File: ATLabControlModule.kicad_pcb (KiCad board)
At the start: 4 copper layers, 44 x 24 mm, 42 parts, among them J1 USB_Type_C_Receptacle, J2 Conn_ARM_SWD_TagConnect_TC2030, SW1 Kailh_Choc_V2_Brown, SW2 Kailh_Choc_V2_Brown, U1 STM32G0B1KEUx, U2 USBLC6-2P6, U3 MIC5317-3.3xM5, U4 SN74LVC1G17DBVRG4

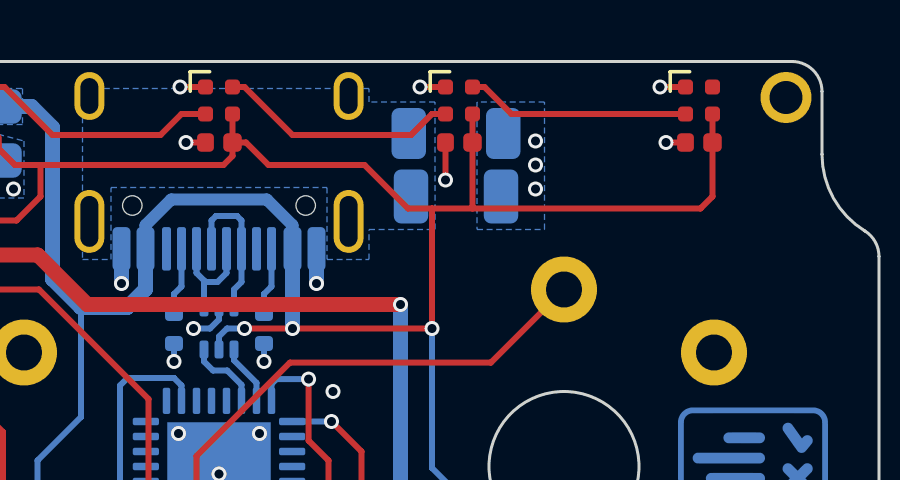
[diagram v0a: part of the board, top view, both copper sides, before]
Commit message: cleanup and add docs
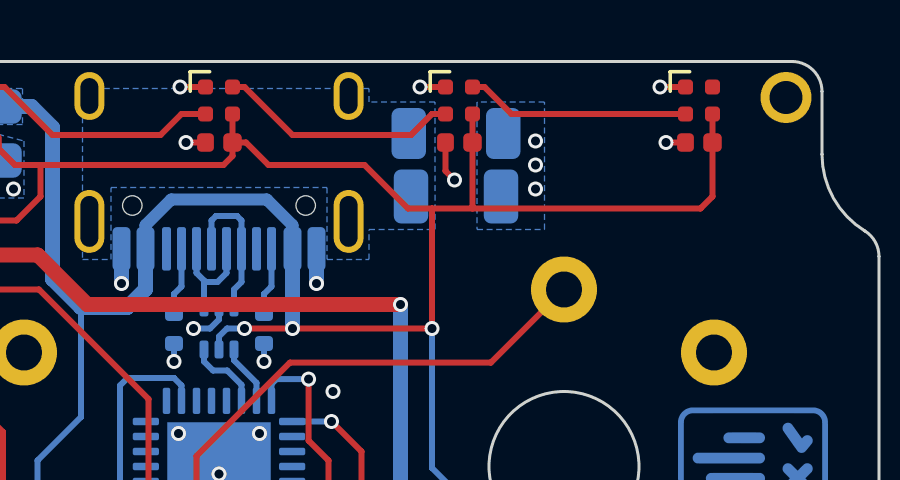
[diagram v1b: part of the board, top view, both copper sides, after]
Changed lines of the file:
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@@
 			)
 		)
-		(property "Datasheet" ""
+		(property "Datasheet" "https://www.lcsc.com/datasheet/C5149201.pdf"
 			(at 0 0 0)
 			(unlocked yes)
@@
 			)
 		)
-		(property "Description" ""
+		(property "Description" "RGB LED with integrated controller"
 			(at 0 0 0)
 			(unlocked yes)
@@
 			)
 		)
+		(property "Manufacturer" "OPSCO Optoelectronics"
+			(at 0 0 180)
+			(unlocked yes)
+			(layer "B.Fab")
+			(hide yes)
+			(effects
+				(font
+					(size 1 1)
+					(thickness 0.15)
+				)
+				(justify mirror)
+			)
+		)
+		(property "Manufacturer Part Number" "SK6812MINI-E"
+			(at 0 0 180)
+			(unlocked yes)
+			(layer "B.Fab")
+			(hide yes)
+			(effects
+				(font
+					(size 1 1)
+					(thickness 0.15)
+				)
+				(justify mirror)
+			)
+		)
+		(property "Distributor" "JLCPCB"
+			(at 0 0 180)
+			(unlocked yes)
+			(layer "B.Fab")
+			(hide yes)
+			(effects
+				(font
+					(size 1 1)
+					(thickness 0.15)
+				)
+				(justify mirror)
+			)
+		)
+		(property "Distributor Part Number" " C5149201"
+			(at 0 0 180)
+			(unlocked yes)
+			(layer "B.Fab")
+			(hide yes)
+			(effects
+				(font
+					(size 1 1)
+					(thickness 0.15)
+				)
+				(justify mirror)
+			)
+		)
 		(property ki_fp_filters "LED?SK6812MINI?E?3.2x2.8mm?P1.5mm*")
 		(sheetname "/")
 		(sheetfile "ATLabControlModule.kicad_sch")
+		(units
+			(unit
+				(name "A")
+				(pins "2" "3" "1" "4")
+			)
+		)
 		(attr smd)
 		(duplicate_pad_numbers_are_jumpers no)
@@
 			)
 		)
-		(property "Manufacturer" ""
+		(property "Manufacturer" "STMicroelectronics"
 			(at 0 0 270)
 			(unlocked yes)
@@
 			)
 		)
-		(property "Manufacturer Part Number" ""
+		(property "Manufacturer Part Number" "STM32G0B1KEU6"
 			(at 0 0 270)
 			(unlocked yes)
@@
 			)
 		)
-		(property "Distributor" ""
+		(property "Distributor" "Digikey"
 			(at 0 0 270)
 			(unlocked yes)
@@
 			)
 		)
-		(property "Distributor Part Number" ""
+		(property "Distributor Part Number" "497-STM32G0B1KEU6-ND"
 			(at 0 0 270)
 			(unlocked yes)
@@
 			)
 		)
-		(property "Datasheet" ""
+		(property "Datasheet" "https://www.lcsc.com/datasheet/C5149201.pdf"
 			(at 0 0 0)
 			(unlocked yes)
@@
 			)
 		)
-		(property "Description" ""
+		(property "Description" "RGB LED with integrated controller"
 			(at 0 0 0)
 			(unlocked yes)
@@
 			)
 		)
+		(property "Manufacturer" "OPSCO Optoelectronics"
+			(at 0 0 180)
+			(unlocked yes)
+			(layer "B.Fab")
+			(hide yes)
+			(effects
+				(font
+					(size 1 1)
+					(thickness 0.15)
+				)
+				(justify mirror)
+			)
+		)
+		(property "Manufacturer Part Number" "SK6812MINI-E"
+			(at 0 0 180)
+			(unlocked yes)
+			(layer "B.Fab")
+			(hide yes)
+			(effects
+				(font
+					(size 1 1)
+					(thickness 0.15)
+				)
+				(justify mirror)
+			)
+		)
+		(property "Distributor" "JLCPCB"
+			(at 0 0 180)
+			(unlocked yes)
+			(layer "B.Fab")
+			(hide yes)
+			(effects
+				(font
+					(size 1 1)
+					(thickness 0.15)
+				)
+				(justify mirror)
+			)
+		)
+		(property "Distributor Part Number" " C5149201"
+			(at 0 0 180)
+			(unlocked yes)
+			(layer "B.Fab")
+			(hide yes)
+			(effects
+				(font
+					(size 1 1)
+					(thickness 0.15)
+				)
+				(justify mirror)
+			)
+		)
 		(property ki_fp_filters "LED?SK6812MINI?E?3.2x2.8mm?P1.5mm*")
 		(sheetname "/")
 		(sheetfile "ATLabControlModule.kicad_sch")
+		(units
+			(unit
+				(name "A")
+				(pins "2" "3" "1" "4")
+			)
+		)
 		(attr smd)
 		(duplicate_pad_numbers_are_jumpers no)
@@
 	)
 	(segment
-		(start 157.15 92.85)
-		(end 157.15 91.7)
-		(width 0.2)
-		(layer "F.Cu")
-		(net "GND")
-	)
-	(segment
 		(start 133.15 92.25)
 		(end 133.15 91.7)
@@
 	)
 	(segment
+		(start 157.15 92.55)
+		(end 157.15 91.7)
+		(width 0.2)
+		(layer "F.Cu")
+		(net "GND")
+	)
+	(segment
 		(start 141.15 92.45)
 		(end 141.85 93.15)
@@
 	)
 	(segment
+		(start 157.45 92.85)
+		(end 157.15 92.55)
+		(width 0.2)
+		(layer "F.Cu")
+		(net "GND")
+	)
+	(segment
 		(start 140.15 89.75)
 		(end 141.15 89.75)
@@
 	)
 	(via
-		(at 157.15 92.85)
+		(at 157.45 92.85)
 		(size 0.5)
 		(drill 0.3)
